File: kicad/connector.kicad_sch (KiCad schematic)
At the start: 1 part, among them J2 Conn_01x06

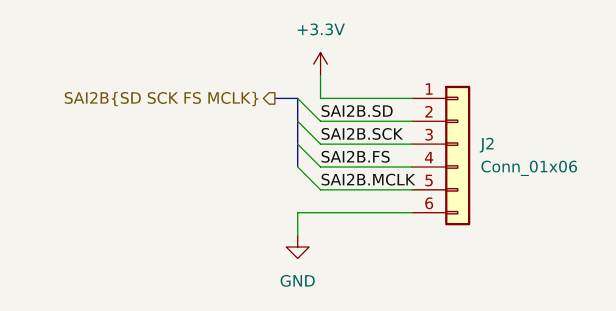
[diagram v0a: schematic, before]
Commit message: journal and readme
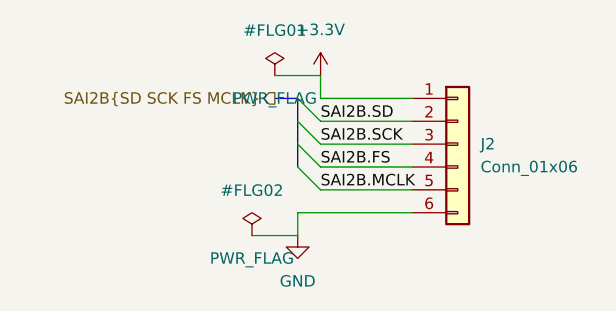
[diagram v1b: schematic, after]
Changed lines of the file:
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@@
+	(wire
+		(pts
+			(xy 58.42 55.88) (xy 63.5 55.88)
+		)
+		(stroke
+			(width 0)
+			(type default)
+		)
+	)
 	(wire
 		(pts
 			(xy 66.04 45.72) (xy 76.2 45.72)
+		)
+		(stroke
+			(width 0)
+			(type default)
+		)
+	)
+	(wire
+		(pts
+			(xy 60.96 38.1) (xy 66.04 38.1)
 		)
 		(stroke
@@
 		)
 	)
+	(symbol
+		(lib_id "power:PWR_FLAG")
+		(at 58.42 55.88 0)
+		(unit 1)
+		(body_style 1)
+		(exclude_from_sim no)
+		(in_bom yes)
+		(on_board yes)
+		(in_pos_files yes)
+		(dnp no)
+		(property "Reference" "#FLG02"
+			(at 58.42 50.88 0)
+			(show_name no)
+			(do_not_autoplace no)
+			(effects
+				(font
+					(size 1.27 1.27)
+				)
+			)
+		)
+		(property "Value" "PWR_FLAG"
+			(at 58.42 58.42 0)
+			(show_name no)
+			(do_not_autoplace no)
+			(effects
+				(font
+					(size 1.27 1.27)
+				)
+			)
+		)
+		(property "Footprint" ""
+			(at 58.42 60.96 0)
+			(hide yes)
+			(show_name no)
+			(do_not_autoplace no)
+			(effects
+				(font
+					(size 1.27 1.27)
+				)
+			)
+		)
+		(property "Datasheet" ""
+			(at 58.42 55.88 0)
+			(show_name no)
+			(do_not_autoplace no)
+			(effects
+				(font
+					(size 1.27 1.27)
+				)
+			)
+		)
+		(property "Description" ""
+			(at 58.42 55.88 0)
+			(show_name no)
+			(do_not_autoplace no)
+			(effects
+				(font
+					(size 1.27 1.27)
+				)
+			)
+		)
+		(pin "1"
+		)
+	)
+	(symbol
+		(lib_id "power:PWR_FLAG")
+		(at 60.96 38.1 0)
+		(unit 1)
+		(body_style 1)
+		(exclude_from_sim no)
+		(in_bom yes)
+		(on_board yes)
+		(in_pos_files yes)
+		(dnp no)
+		(property "Reference" "#FLG01"
+			(at 60.96 33.1 0)
+			(show_name no)
+			(do_not_autoplace no)
+			(effects
+				(font
+					(size 1.27 1.27)
+				)
+			)
+		)
+		(property "Value" "PWR_FLAG"
+			(at 60.96 40.64 0)
+			(show_name no)
+			(do_not_autoplace no)
+			(effects
+				(font
+					(size 1.27 1.27)
+				)
+			)
+		)
+		(property "Footprint" ""
+			(at 60.96 43.18 0)
+			(hide yes)
+			(show_name no)
+			(do_not_autoplace no)
+			(effects
+				(font
+					(size 1.27 1.27)
+				)
+			)
+		)
+		(property "Datasheet" ""
+			(at 60.96 38.1 0)
+			(show_name no)
+			(do_not_autoplace no)
+			(effects
+				(font
+					(size 1.27 1.27)
+				)
+			)
+		)
+		(property "Description" ""
+			(at 60.96 38.1 0)
+			(show_name no)
+			(do_not_autoplace no)
+			(effects
+				(font
+					(size 1.27 1.27)
+				)
+			)
+		)
+		(pin "1"
+		)
+	)
